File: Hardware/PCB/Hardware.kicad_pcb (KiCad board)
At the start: 2 copper layers, 68.6 x 53.3 mm, 36 parts, among them J1 Conn_01x03_Male, M1 Motor_Servo, M2 Motor_Servo, M3 Motor_Servo, P1 Power, P2 Analog, P3 Digital, P4 Digital, P5 CONN_01X01, P6 CONN_01X01, P7 CONN_01X01, P8 CONN_01X01, U1 HC-SR04, U2 HC-SR04, U3 HC-SR04

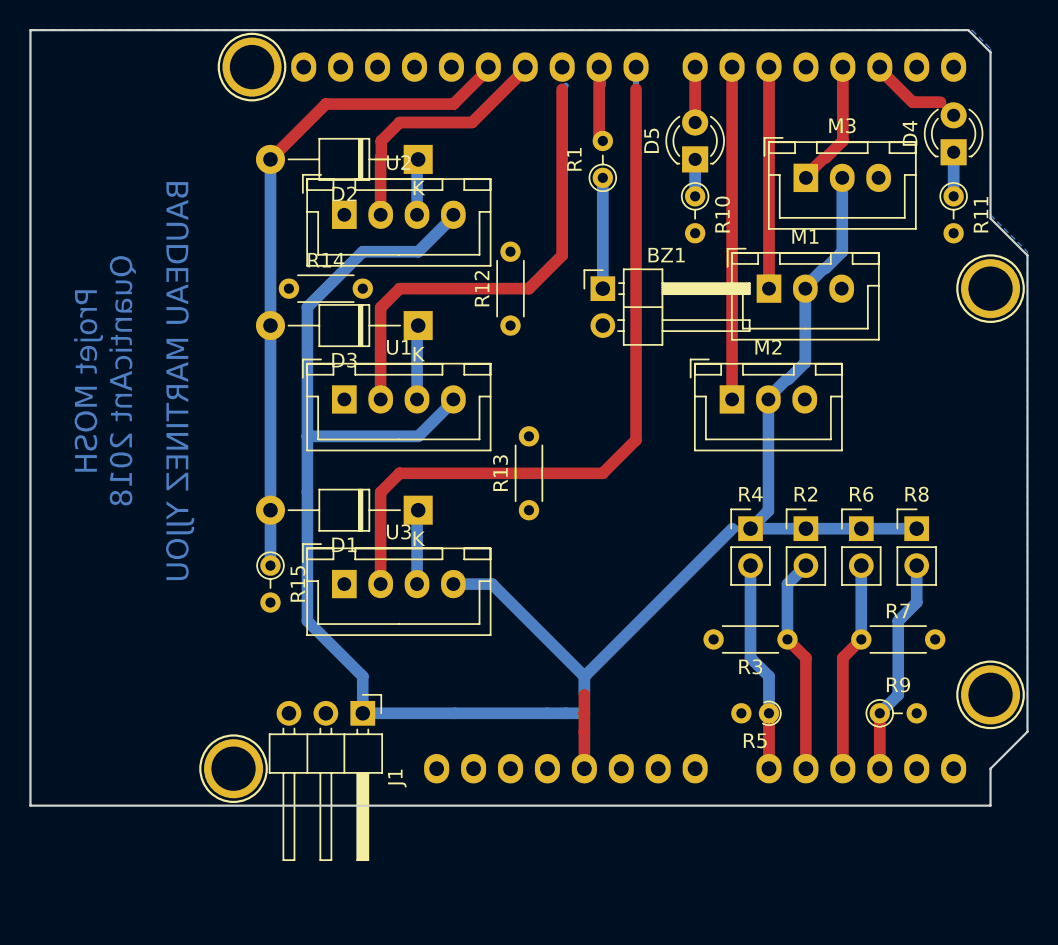
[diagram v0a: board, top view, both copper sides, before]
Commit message: PCB final
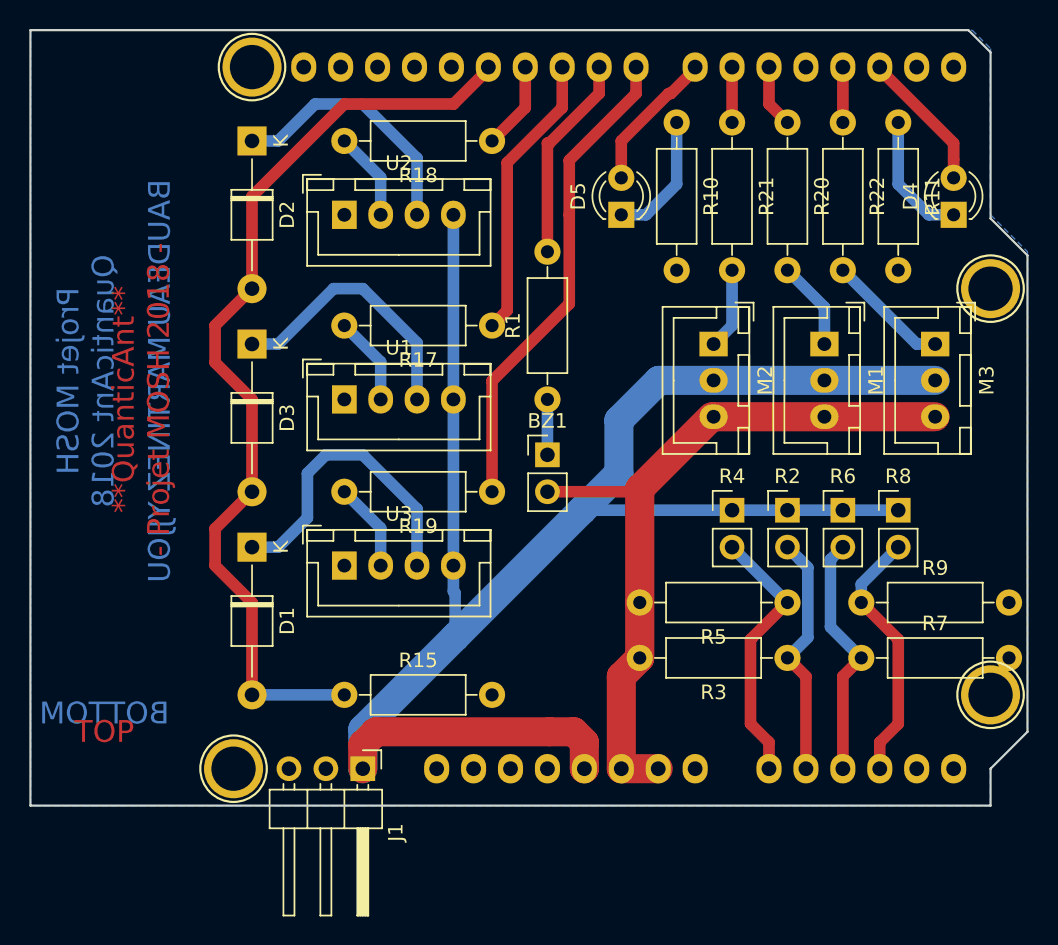
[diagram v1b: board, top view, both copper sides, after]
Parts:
- removed R12, R13, R14: R, Resistor_THT:R_Axial_DIN0204_L3.6mm_D1.6mm_P5.08mm_Horizontal
- added R17: R, Resistor_THT:R_Axial_DIN0207_L6.3mm_D2.5mm_P10.16mm_Horizontal, F.Cu at (142.7, 93.3)
- added R18: R, Resistor_THT:R_Axial_DIN0207_L6.3mm_D2.5mm_P10.16mm_Horizontal, F.Cu at (142.7, 80.6)
- added R19: R, Resistor_THT:R_Axial_DIN0207_L6.3mm_D2.5mm_P10.16mm_Horizontal, F.Cu at (142.7, 104.8)
- added R20: R, Resistor_THT:R_Axial_DIN0207_L6.3mm_D2.5mm_P10.16mm_Horizontal, F.Cu at (163.1, 79.4)
- added R21: R, Resistor_THT:R_Axial_DIN0207_L6.3mm_D2.5mm_P10.16mm_Horizontal, F.Cu at (159.3, 79.4)
- added R22: R, Resistor_THT:R_Axial_DIN0207_L6.3mm_D2.5mm_P10.16mm_Horizontal, F.Cu at (166.9, 79.4)
- BZ1: footprint Connector_PinHeader_2.54mm:PinHeader_1x02_P2.54mm_Horizontal -> Connector_PinHeader_2.54mm:PinHeader_1x02_P2.54mm_Vertical
- R1, R10, R11, R15, R9: footprint Resistor_THT:R_Axial_DIN0204_L3.6mm_D1.6mm_P2.54mm_Vertical -> Resistor_THT:R_Axial_DIN0207_L6.3mm_D2.5mm_P10.16mm_Horizontal
- R3, R7: footprint Resistor_THT:R_Axial_DIN0204_L3.6mm_D1.6mm_P5.08mm_Horizontal -> Resistor_THT:R_Axial_DIN0207_L6.3mm_D2.5mm_P10.16mm_Horizontal
- R5: footprint Resistor_THT:R_Axial_DIN0204_L3.6mm_D1.6mm_P1.90mm_Vertical -> Resistor_THT:R_Axial_DIN0207_L6.3mm_D2.5mm_P10.16mm_Horizontal
- moved R1 15.7 mm to (146.6, 98.4)
- moved M3 14.5 mm to (173.2, 94.6), turned to 270 degrees
- moved BZ1 12.0 mm to (146.6, 102.2)
- moved D1 11.7 mm to (126.2, 108.6), turned to 270 degrees
- moved D2 11.5 mm to (126.2, 80.6), turned to 270 degrees
- moved D3 11.5 mm to (126.2, 94.6), turned to 270 degrees
- moved R15 10.2 mm to (132.6, 118.7), turned to 0 degrees
- moved R5 7.73 mm to (163.1, 112.4)
- moved R9 7.73 mm to (168.1, 112.4)
- moved R11 6.35 mm to (170.7, 79.4)
- moved D5 6.35 mm to (151.6, 85.7)
- moved M1 5.39 mm to (165.6, 94.6), turned to 270 degrees
- moved R10 5.24 mm to (155.4, 79.4)
- moved D4 4.30 mm to (174.5, 85.7)
- moved M2 4.02 mm to (158.0, 94.6), turned to 270 degrees
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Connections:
- M1 pad 1: /5(**) -> Net-(M1-Pad1)
- M2 pad 1: /6(**) -> Net-(M2-Pad1)
- M3 pad 1: /3(**) -> Net-(M3-Pad1)
- P3 pad 1: /A5(SCL) -> Net-(P3-Pad1)
- P3 pad 2: /A4(SDA) -> Net-(P3-Pad2)
- U1 pad 2: /10(**/SS) -> Net-(R17-Pad2)
- U2 pad 2: /11(**/MOSI) -> Net-(R18-Pad2)
- U3 pad 2: /8 -> Net-(R19-Pad2)
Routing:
- net GND: track 0.00 -> 51.1 mm
- net +5V: track 146.8 -> 125.2 mm
- net /8: track 52.7 -> 33.3 mm
- net /12(MISO): track 45.6 -> 64.9 mm
- net /6(**): track 22.9 -> 3.81 mm
- net Net-(D1-Pad1): track 5.24 -> 21.2 mm
- net Net-(D2-Pad1): track 4.08 -> 18.1 mm
- net Net-(D3-Pad1): track 5.24 -> 18.5 mm
- net /10(**/SS): track 32.4 -> 19.9 mm
- net /5(**): track 15.2 -> 4.34 mm
- net /11(**/MOSI): track 17.4 -> 6.52 mm
- net Net-(M3-Pad1): track 0.00 -> 8.45 mm
- net /9(**): track 6.56 -> 14.8 mm
- net Net-(D5-Pad1): track 2.54 -> 8.92 mm
- net Net-(R18-Pad2): track 0.00 -> 6.30 mm
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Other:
- net class Default: trace_width 0.5 -> 0.8
- board text added: "**QuanticAnt** - Projet MOSH 2018 -"
- board text added: "BOTTOM"
- board text added: "TOP"
